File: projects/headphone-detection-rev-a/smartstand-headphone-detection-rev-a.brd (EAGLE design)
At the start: 22 x 23 mm, 19 parts, among them J1 T1M-5POS, U1 VL6180XV0NR, U2 LP5907MFX-2.8, U3 BSS138, U4 BSS138

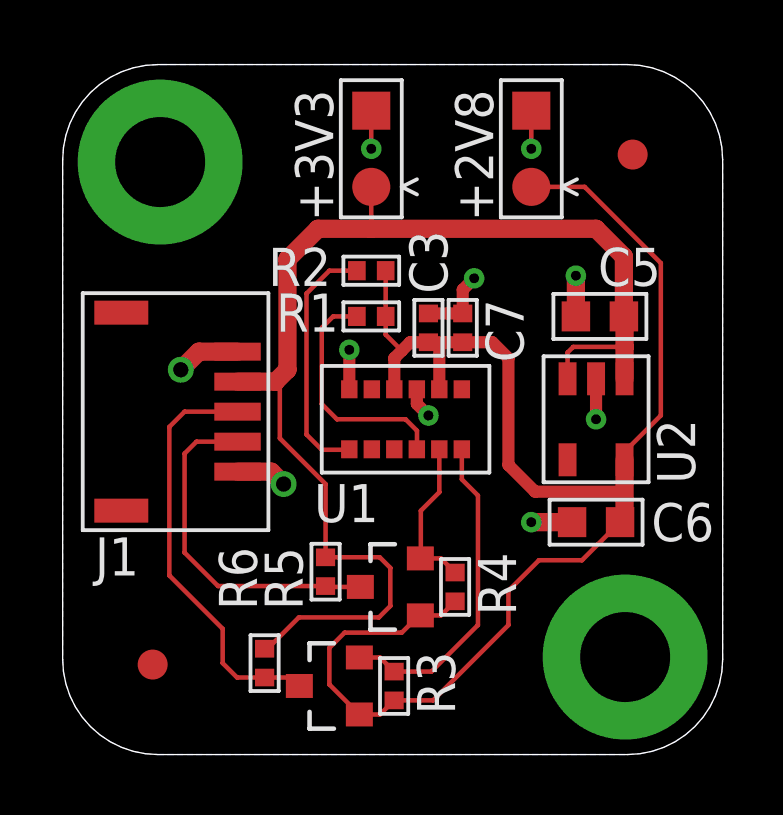
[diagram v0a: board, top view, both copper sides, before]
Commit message: Adding part numbers to schematic.
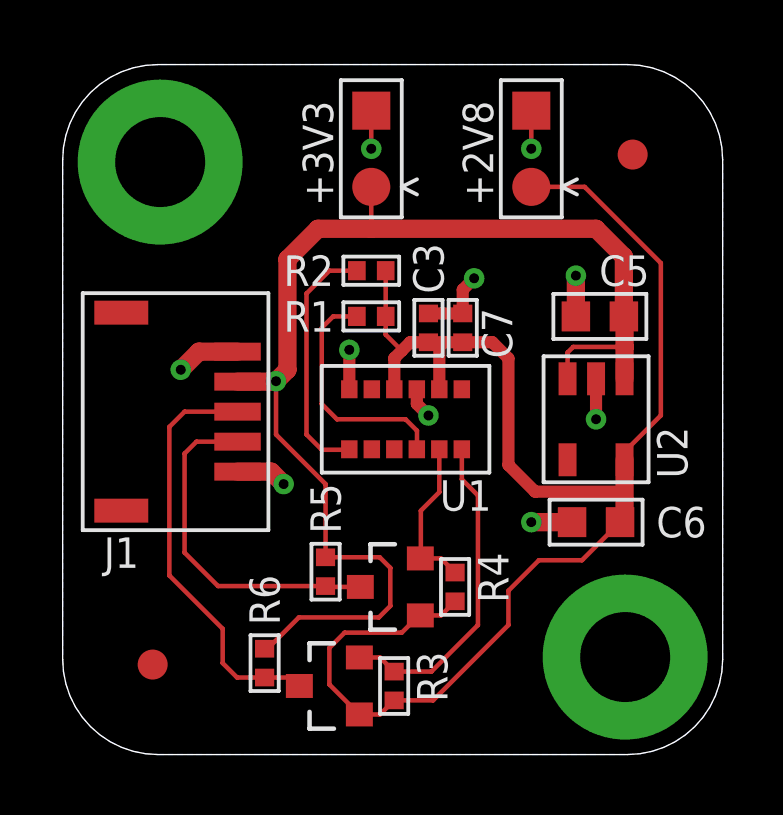
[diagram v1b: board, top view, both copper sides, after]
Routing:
- net +3V3: track 40.8 -> 41.0 mm, vias 0 -> 1
